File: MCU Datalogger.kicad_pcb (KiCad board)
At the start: 2 copper layers, 51.2 x 36 mm, 29 parts, among them J1 Conn_01x04_Pin, J2 Conn_01x09_Pin, J3 Conn_01x04_Pin, J4 Conn_02x03_Odd_Even, U1 24LC1025, U2 DS1337S_, U3 24LC1025, U4 ATMEGA328P-AU, Y1 32.768 KHz, Y2 16 MHz

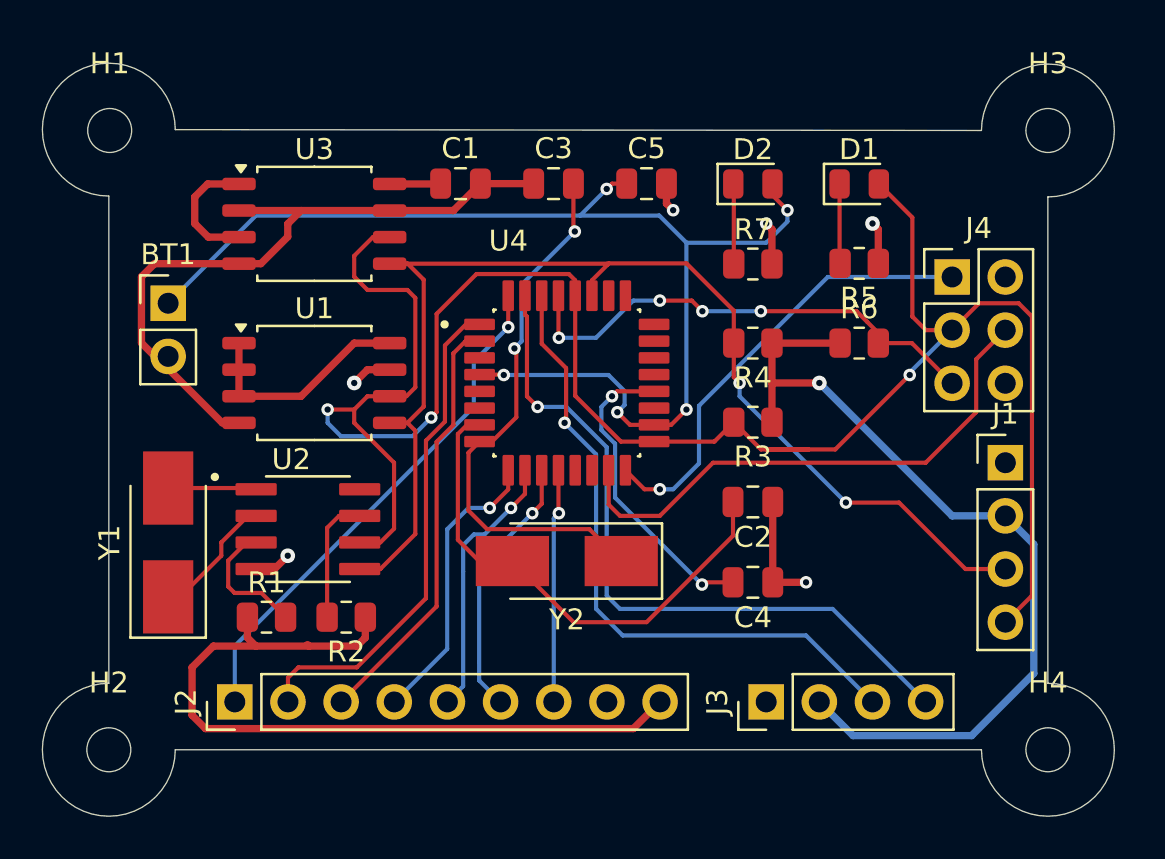
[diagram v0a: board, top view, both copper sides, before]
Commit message: Completed routing.
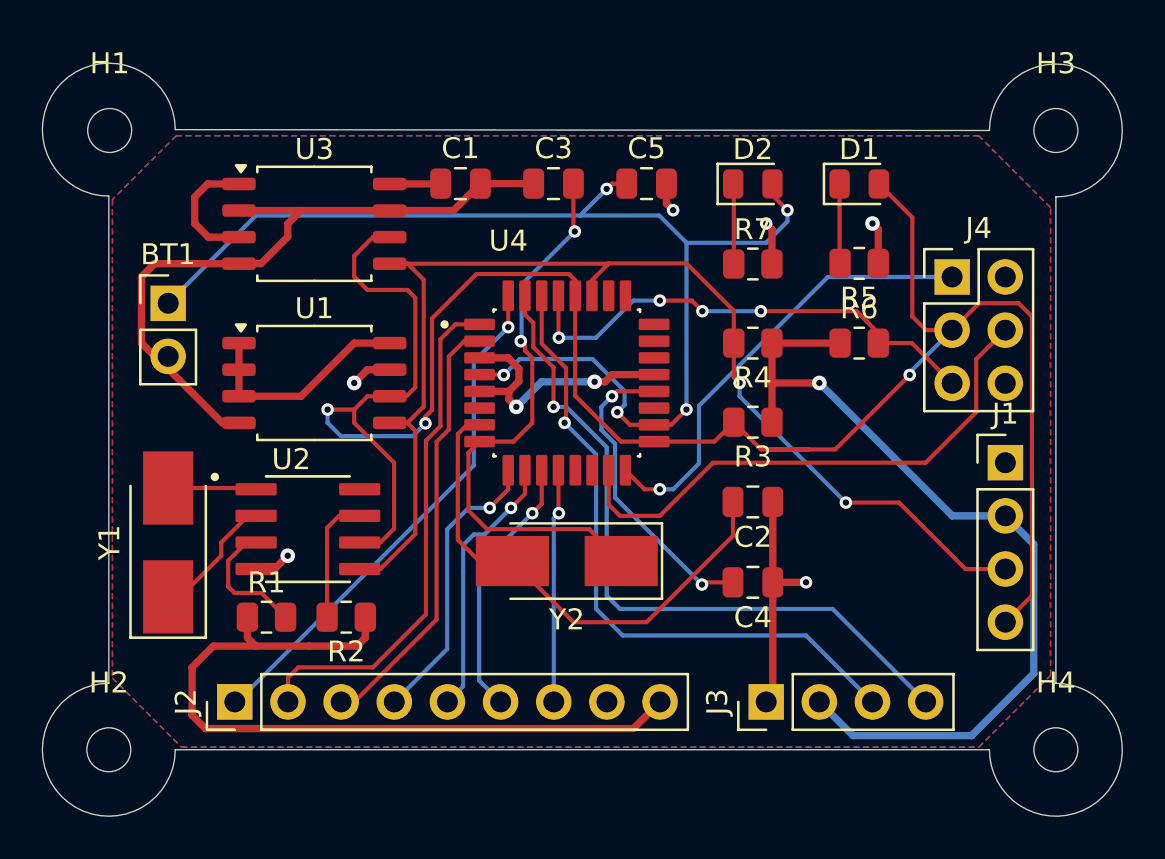
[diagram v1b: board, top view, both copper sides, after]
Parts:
- moved H3 0.38 mm to (200.5, 86.4)
- moved H4 0.38 mm to (200.5, 116.0)
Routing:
- net GND: track 48.9 -> 67.7 mm, vias 6 -> 8
- net Net-(U4-PB7): track 26.5 -> 27.5 mm
- net /D3: track 23.8 -> 24.6 mm
- net Net-(BT1-+): track 57.5 -> 58.1 mm
- added copper zone on F.Cu, net /Vcc
- added copper zone on B.Cu, net GND
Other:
- board size 51.2 x 36 mm -> 51.6 x 36 mm
